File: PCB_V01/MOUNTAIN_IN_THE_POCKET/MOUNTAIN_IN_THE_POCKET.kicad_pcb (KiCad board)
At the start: 2 copper layers, 61 parts, among them IC1 AZ1117CH-3.3TRG1, J1 CON_ALIM, Q2 2N7002, SW1 SW_MEC_5E, SW2 SW_MEC_5E, U1 AP63205WU, U2 AS1115-BSST

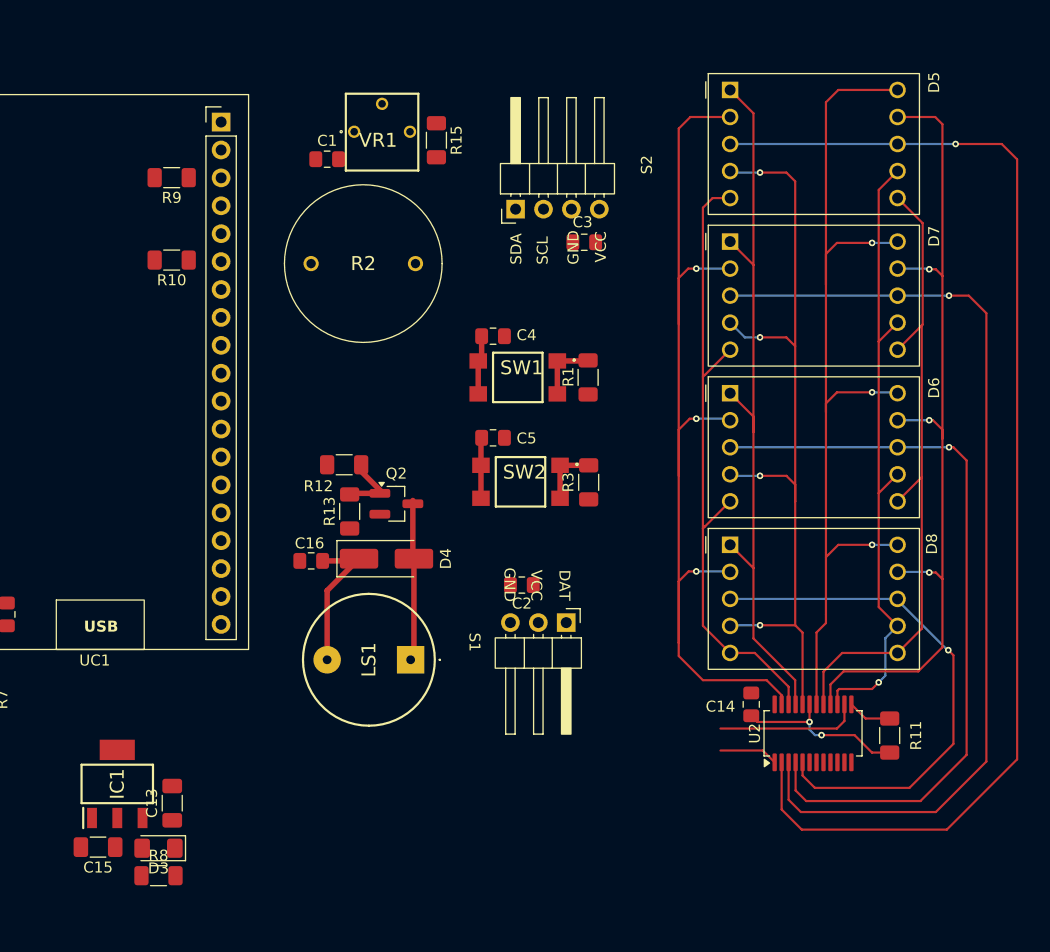
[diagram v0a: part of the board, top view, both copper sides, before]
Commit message: actualizado routing
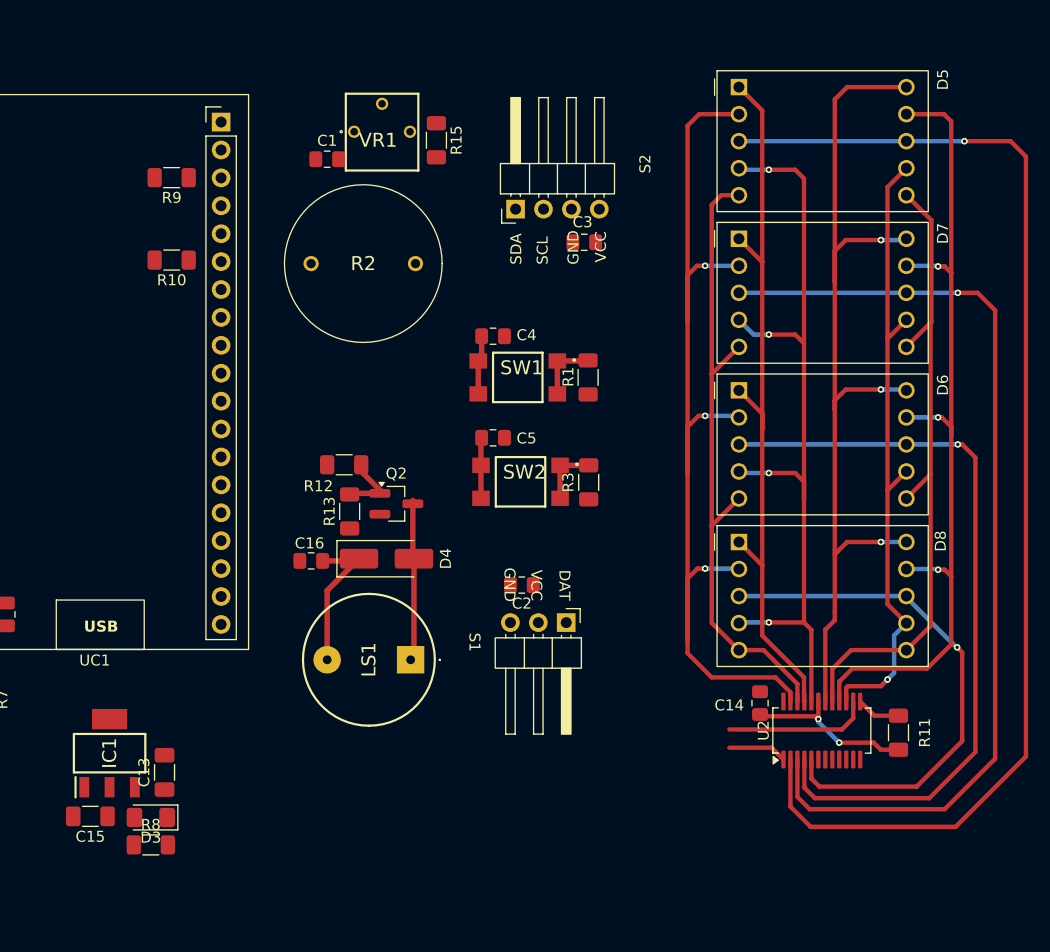
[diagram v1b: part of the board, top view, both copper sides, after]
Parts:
- moved C13 2.89 mm to (107.6, 96.7)
- moved C15 2.89 mm to (100.8, 100.7)
- moved D3 2.89 mm to (106.3, 100.8)
- moved IC1 2.89 mm to (102.6, 94.9)
- moved R8 2.89 mm to (106.3, 103.2)
- moved R11 0.84 mm to (174.4, 93.0)
- moved D5 0.84 mm to (159.9, 34.3)
- moved D6 0.84 mm to (159.9, 61.9)
- moved D7 0.84 mm to (159.9, 48.1)
- moved D8 0.84 mm to (159.9, 75.7)
- moved U2 0.84 mm to (167.4, 92.8)
- moved C14 0.81 mm to (161.8, 90.3)
